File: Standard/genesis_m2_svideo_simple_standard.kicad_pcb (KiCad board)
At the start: 2 copper layers, 33.3 x 16.9 mm, 11 parts, among them J1 Y In, J2 C In, J3 Y Out, J4 C Out, J5 GND, J6 YGND, J7 CGND

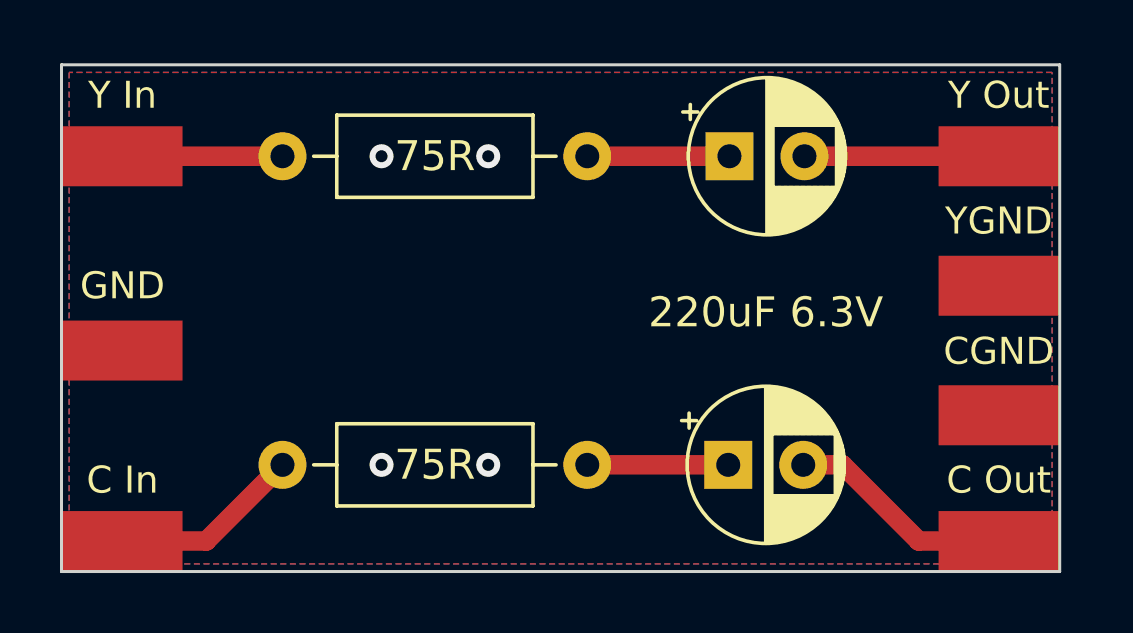
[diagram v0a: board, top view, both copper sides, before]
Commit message: standard - minor update
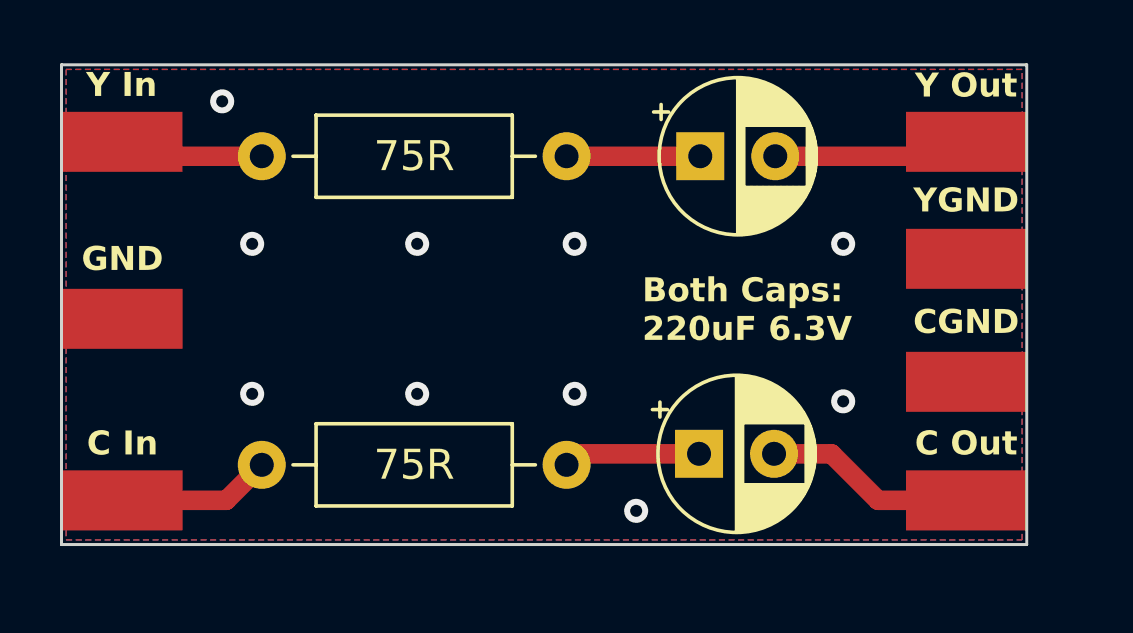
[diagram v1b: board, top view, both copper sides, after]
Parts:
- moved J4 1.74 mm to (102.8, 80.0)
- moved J7 1.56 mm to (102.8, 76.1)
- moved J6 1.41 mm to (102.8, 72.0)
- moved J2 1.36 mm to (74.7, 80.0)
- moved J3 1.19 mm to (102.8, 68.1)
- moved J5 1.06 mm to (74.7, 74.0)
- moved C2 1.04 mm to (93.9, 78.5)
- moved C1 0.97 mm to (93.9, 68.6)
- moved R1 0.69 mm to (79.3, 68.6)
- moved R2 0.69 mm to (79.3, 78.9)
- moved J1 0.48 mm to (74.7, 68.1)
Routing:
- net Net-(J2-Pin_1): track 6.39 -> 5.13 mm
- net Net-(J4-Pin_1): track 7.57 -> 7.04 mm
- net GND: vias 4 -> 10
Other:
- board size 33.3 x 16.9 mm -> 32.2 x 16 mm
- board text added: "Both Caps: 220uF 6.3V"
- board text removed: "Y = Luma C = Chroma"
